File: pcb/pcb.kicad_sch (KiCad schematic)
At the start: 49 parts, among them J1 GPIO, J2 3.3V Power, J3 3.3V Power, J4 SPI2, J5 SWD, J6 5V Power, J7 5V Power, J8 I2C2, J9 USART1, SW1 SW_Push, SW2 SW_SPDT, SW3 SW_SPDT, U1 STM32F103C8T6, U2 AMS1117-3.3, Y1 8MHz

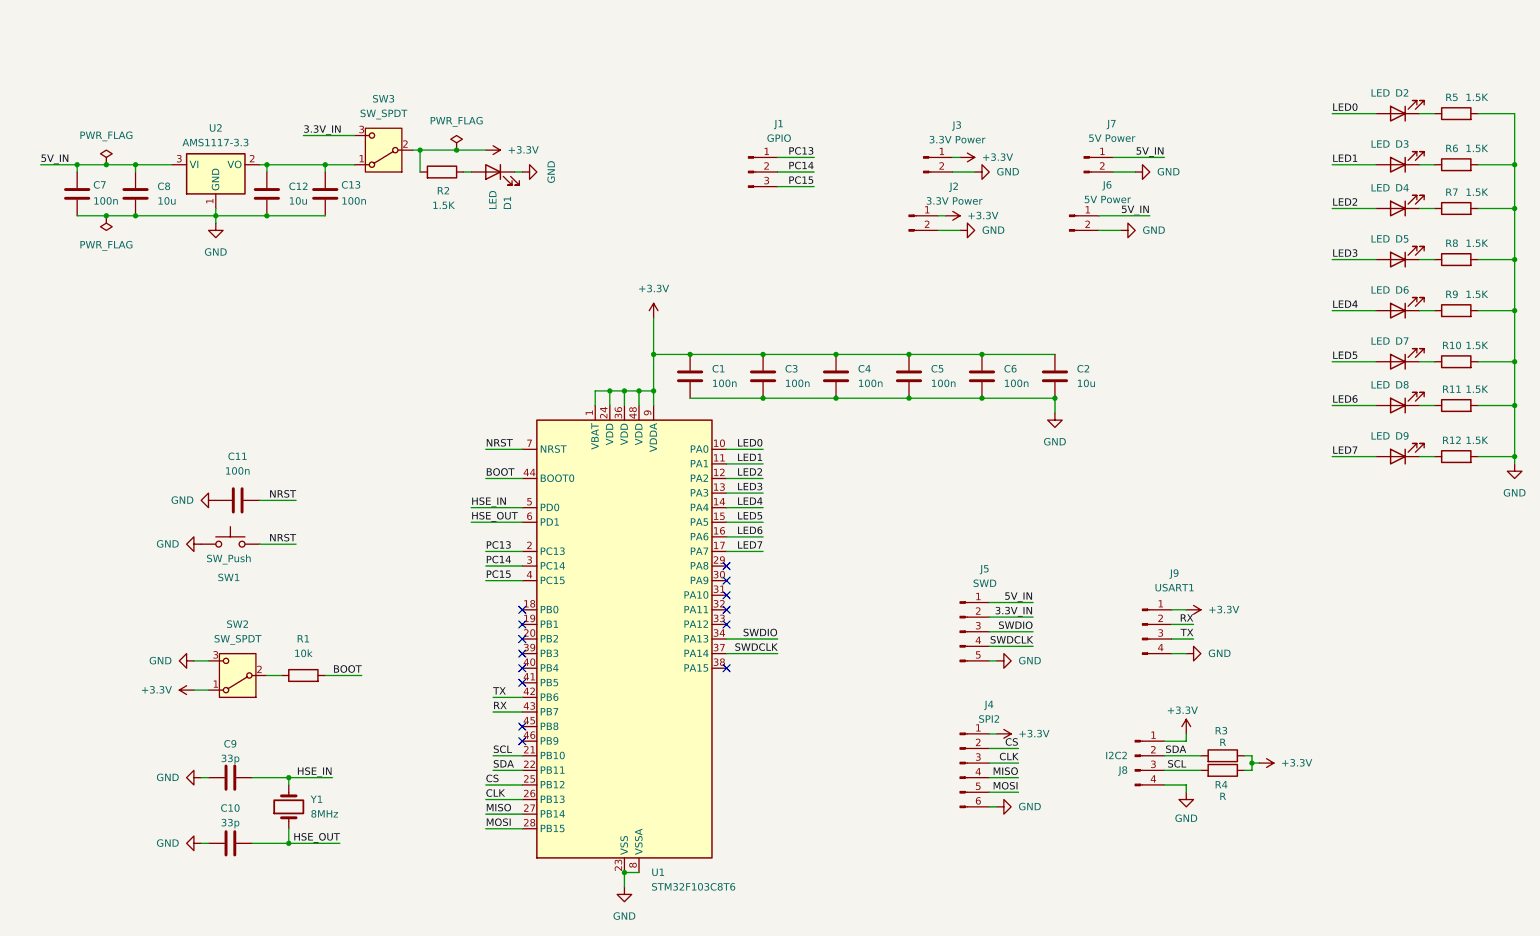
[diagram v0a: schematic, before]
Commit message: Cleaned up the schematics
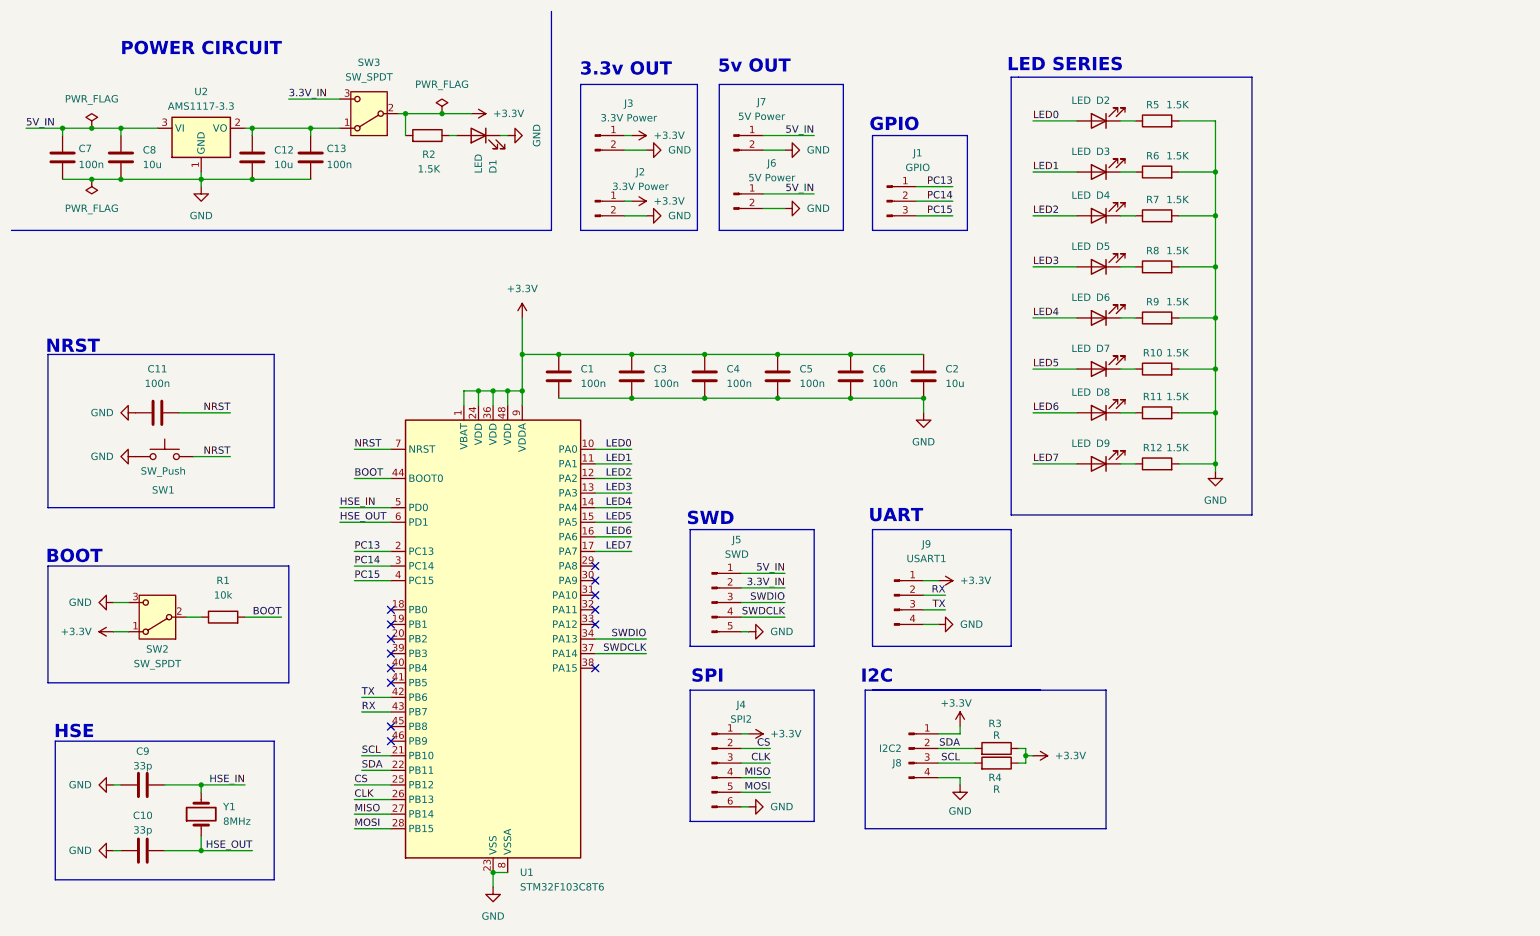
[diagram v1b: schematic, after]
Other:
- note added: "3.3v OUT"
- note added: "5v OUT"
- note added: "BOOT"
- note added: "GPIO"
- note added: "HSE"
- note added: "I2C"
- note added: "LED SERIES"
- note added: "NRST"
- note added: "POWER CIRCUIT"
- note added: "SPI"
- note added: "SWD"
- note added: "UART"
- moved on the sheet: C1, C10, C11, C12, C13, C2, C3, C4, C5, C6, C7, C8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
